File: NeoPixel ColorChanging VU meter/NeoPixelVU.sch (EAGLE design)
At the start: 12 parts, among them IC1 LM324N

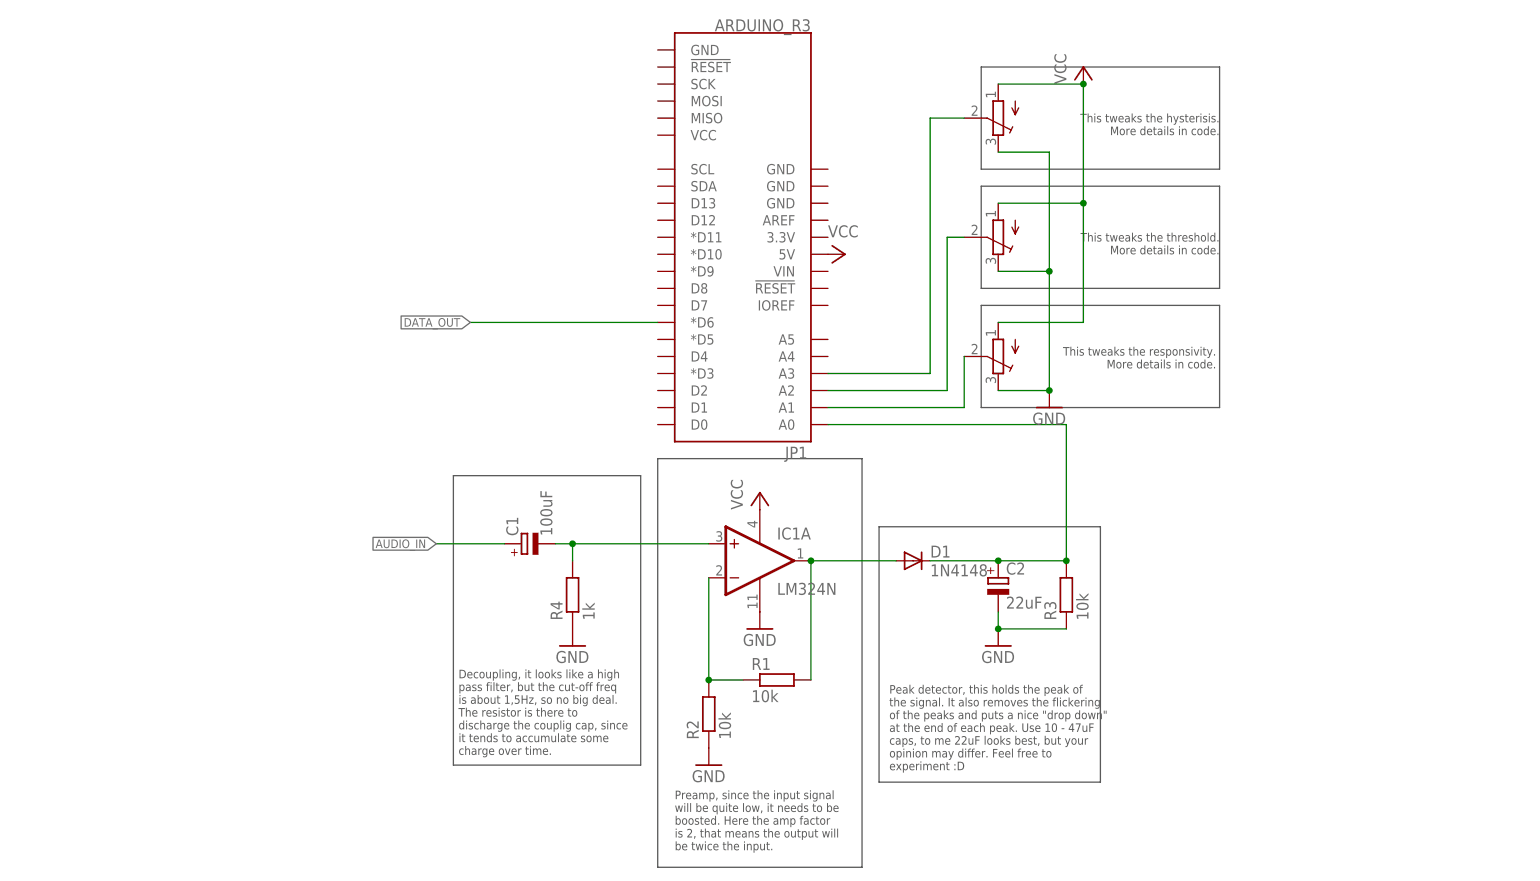
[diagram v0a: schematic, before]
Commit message: Add files via upload
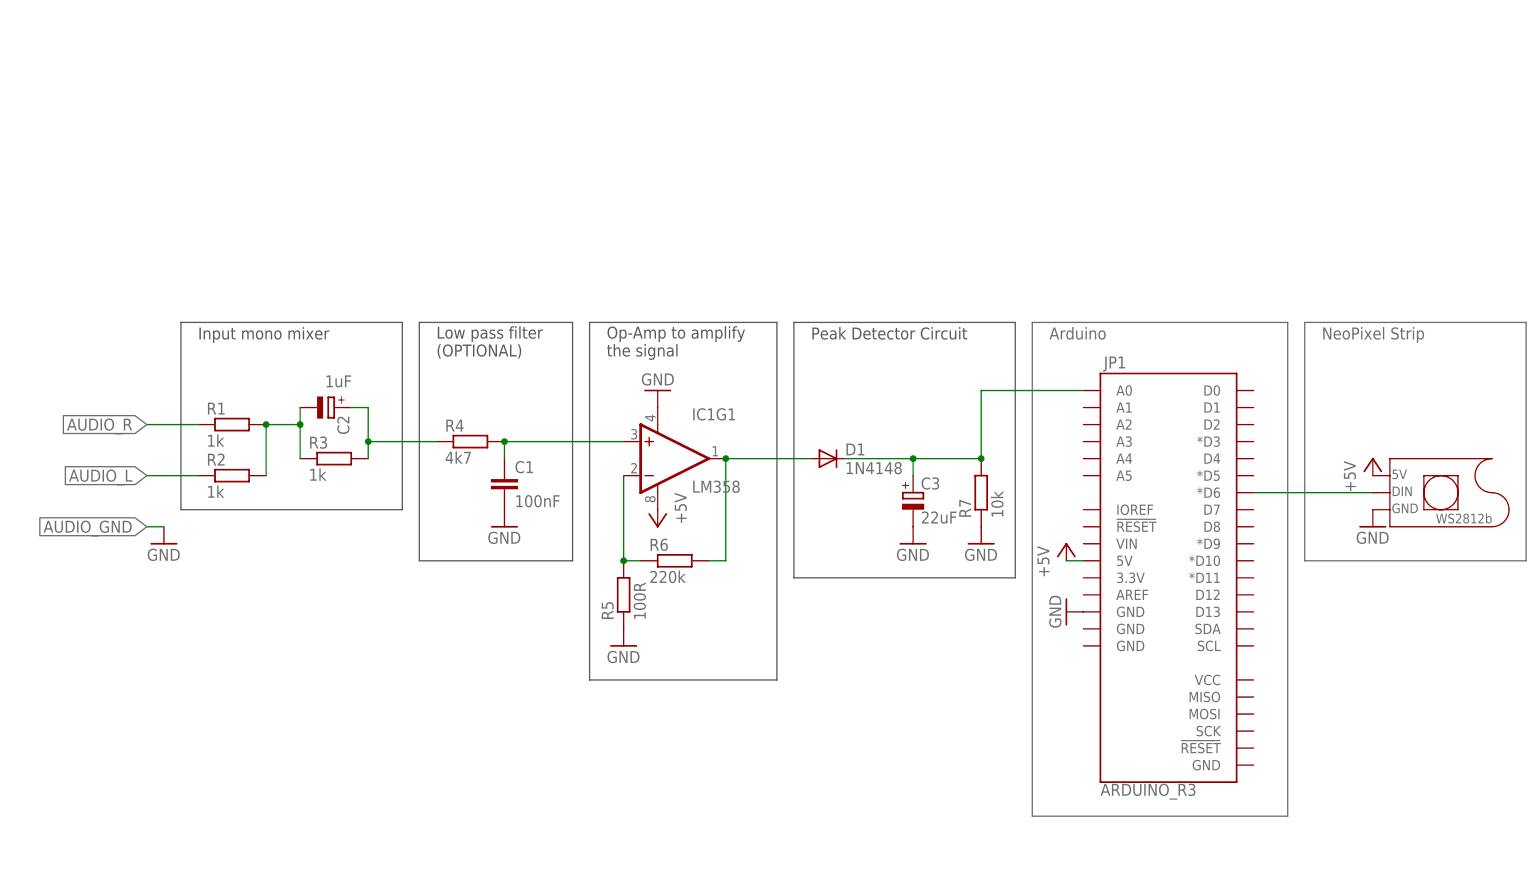
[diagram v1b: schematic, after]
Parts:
- removed U$1, U$2, U$3: (no value), adafruit:TRIMPOTTC33X
- added C3: 22uF, rcl:CPOL-EU085CS-1AR
- added R5: 100R, rcl:R-EU_0411/3V
- added R6: 220k, rcl:R-EU_0411/3V
- added R7: 10k, rcl:R-EU_0411/3V
- C1: value 100uF -> 100nF; device rcl:CPOL-EU153CLV-1010 -> rcl:C-EU025-024X044
- C2: value 22uF -> 1uF; device rcl:CPOL-EU153CLV-1010 -> rcl:CPOL-EU085CS-1AR
- IC1: value LM324N -> LM358; device linear:LM324N -> SparkFun-AnalogIC:LM358
- R1, R2, R3: value 10k -> 1k; device rcl:R-EU_0309/10 -> rcl:R-EU_0411/3V
- R4: value 1k -> 4k7; device rcl:R-EU_0309/10 -> rcl:R-EU_0411/3V
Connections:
- net DATA_OUT renamed N$1
- removed net AUDIO_IN: C1.+
- removed net N$1 (its old number): IC1A.-IN, R1.1, R2.2
- removed net VCC: IC1P.V+, JP1.5V, U$1.A, U$2.A, U$3.A
- new net +5V: IC1G1.V+, JP1.5V
- new net AUDIO_L: R2.1
- new net AUDIO_R: R1.1
- net GND: now also C1.2, C3.-, IC1G1.V-, JP1.GND@2, R5.1, R7.1; no longer C2.-, IC1P.V-, R2.1, R3.1, R4.1, U$1.E, U$2.E, U$3.E
- net N$2: now also C2.+, R3.2, R4.1; no longer C1.-, IC1A.+IN, R4.2
- net N$3: now also C1.1, IC1G1.+IN, R4.2; no longer D1.A, IC1A.OUT, R1.2
- net N$4: now also IC1G1.-IN, R5.2, R6.1; no longer C2.+, D1.C, JP1.A0, R3.2
- net N$5: now also C2.-, R1.2, R2.2, R3.1; no longer JP1.A1, U$2.S
- net N$6: now also D1.A, IC1G1.OUT, R6.2; no longer JP1.A2, U$1.S
- net N$7: now also C3.+, D1.C, JP1.A0, R7.2; no longer JP1.A3, U$3.S
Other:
- note added: "5V"
- note added: "Arduino"
- note added: "DIN"
- note added: "GND"
- note added: "Input mono mixer"
- note added: "Low pass filter (OPTIONAL)"
- note added: "NeoPixel Strip"
- note added: "Op-Amp to amplify the signal"
- note added: "Peak Detector Circuit"
- note added: "WS2812b"
- note removed: "Decoupling, it looks like a high pass filter, but the cut-off freq is about 1,5Hz, so no big deal. The resistor is there to discharge the couplig cap, since it tends to accumulate some charge over time."
- note removed: "Peak detector, this holds the peak of the signal. It also removes the flickering of the peaks and puts a nice "drop down" at the end of each peak. Use 10 - 47uF caps, to me 22uF looks best, but your opinion may differ. Feel free to experiment :D"
- note removed: "Preamp, since the input signal will be quite low, it needs to be boosted. Here the amp factor is 2, that means the output will be twice the input."
- note removed: "This tweaks the hysterisis. More details in code."
- note removed: "This tweaks the responsivity. More details in code."
- note removed: "This tweaks the threshold. More details in code."
- moved on the sheet: C2, D1, JP1, R1, R2, R3, R4
